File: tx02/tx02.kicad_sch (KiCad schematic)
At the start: 13 parts, among them J1 USB-C, J2 OUT, SW1 SW_Push, SW2 SW_SPDT, U1 ATtiny202-SS, U2 CH340K

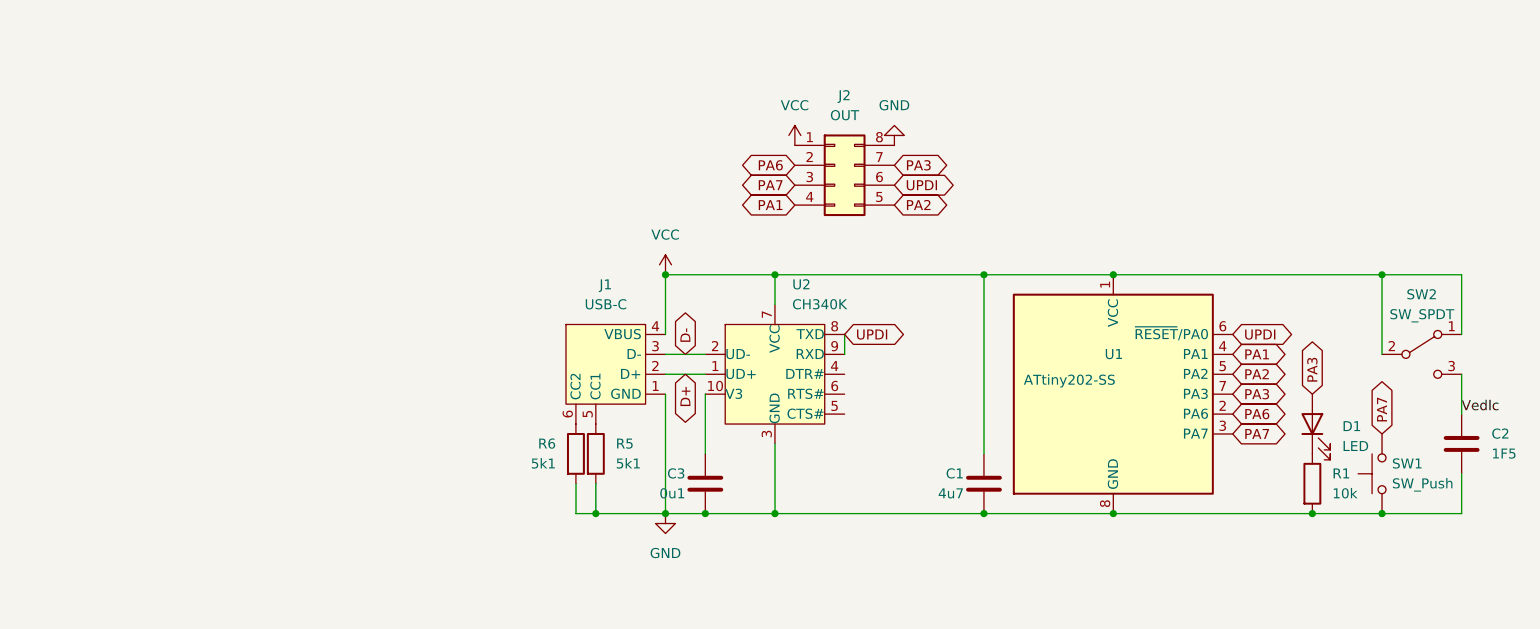
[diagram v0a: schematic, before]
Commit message: -
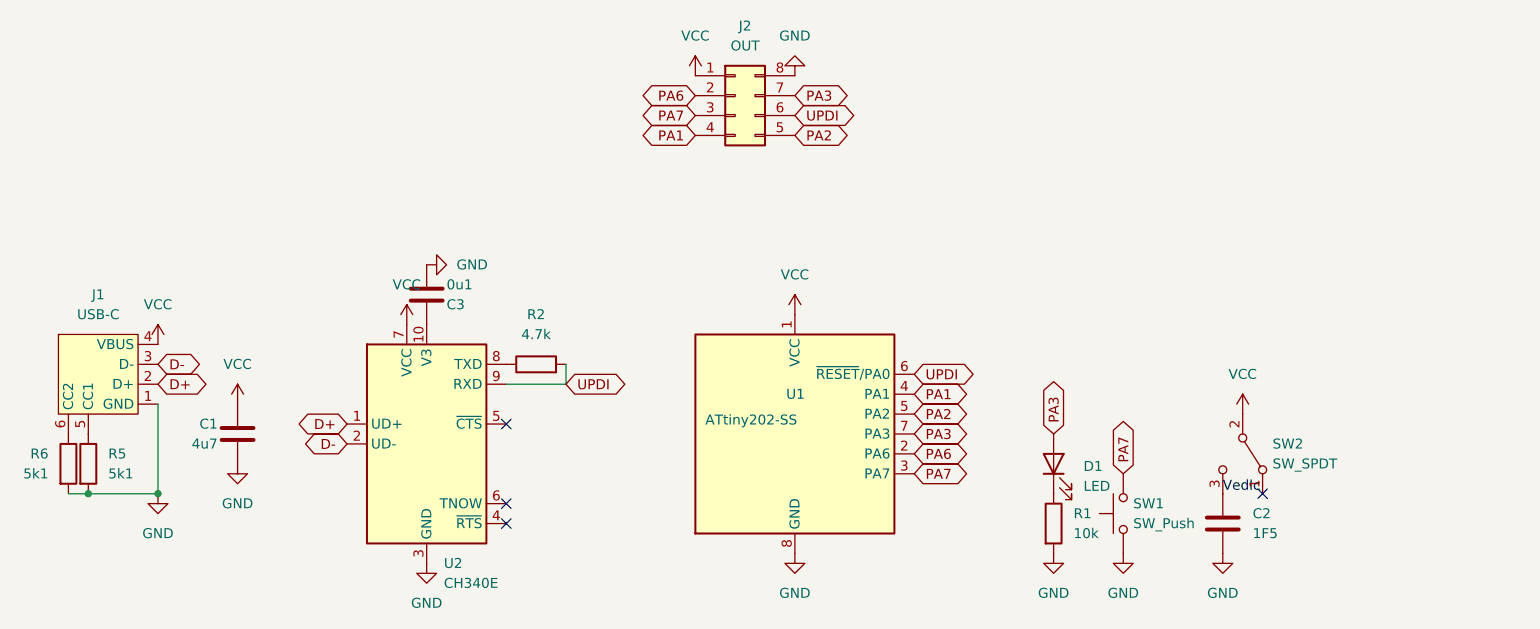
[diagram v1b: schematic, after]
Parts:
- removed U2: CH340K, Package_SO:SSOP-10_3.9x4.9mm_P1.00mm, symbol Library:CH340K
- added R2: 4.7k, Resistor_SMD:R_0603_1608Metric, symbol Device:R
- added U2: CH340E, Package_SO:MSOP-10_3x3mm_P0.5mm, symbol Interface_USB:CH340E
- SW1: footprint Library:sw_push_smd -> Library:alps-skrp
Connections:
- net D+: now also U2.1 (UD+)
- net D-: now also U2.2 (UD-)
- net GND: now also U2.3 (GND)
- net UPDI: now also R2.2, U2.9 (RXD)
- net VCC: now also U2.7 (VCC); no longer SW2.1 (A)
- net at C3.1: now also U2.10 (V3)
- new net: R2.1, U2.8 (TXD)
- no-connect marks 0 -> 4
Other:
- moved on the sheet: C1, C2, D1, J1, J2, R1, R5, R6, SW1, SW2, U1
